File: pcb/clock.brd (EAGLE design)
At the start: 145 x 50 mm, 76 parts, among them IC1 STM32F072C8T6, IC2 REG1117, IC3 24C64ST, SW1 324_SW324_SWITCH_FOOT_HOLE, SW4 324_SW324_SWITCH_FOOT_HOLE, U1 DS18B20, U2 USBC_16P, X2 32.768KHz

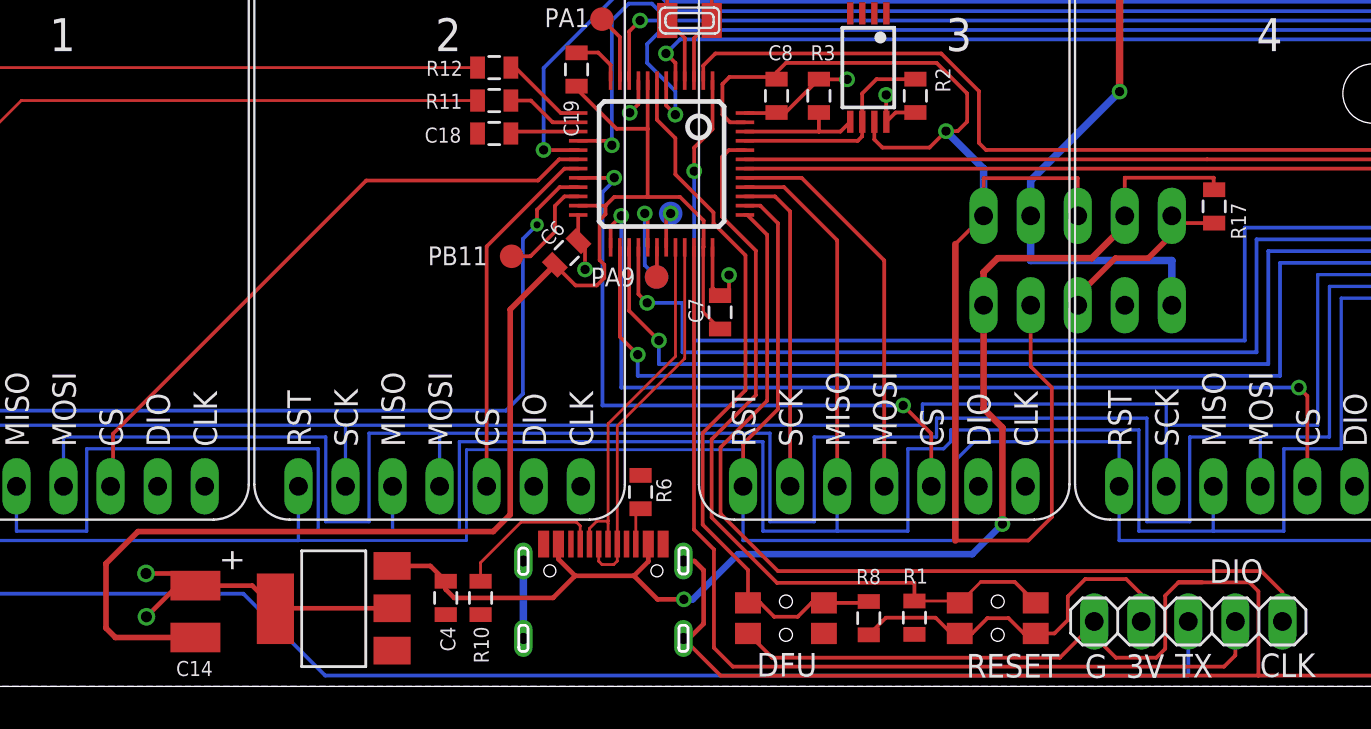
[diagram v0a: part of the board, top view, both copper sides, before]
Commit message: clean up
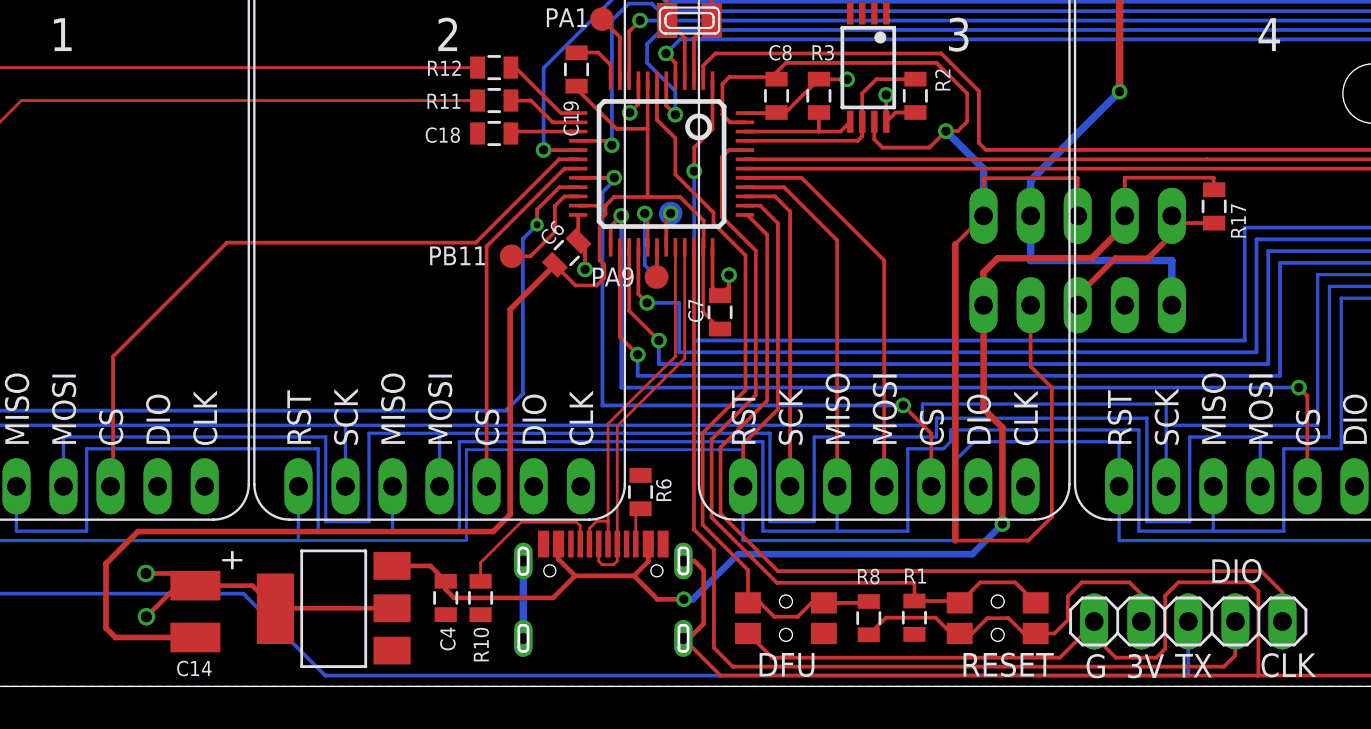
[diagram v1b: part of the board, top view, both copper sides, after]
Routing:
- net EXIXE1_CS: track 34.1 -> 36.6 mm
- net GND: track 277.5 -> 276.2 mm
- net +3V3: track 157.3 -> 156.7 mm
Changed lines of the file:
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@@
 <text x="79.756" y="5.588" size="1.27" layer="25">DIO</text>
 <text x="85.471" y="1.778" size="1.27" layer="25" rot="R180">CLK</text>
-<text x="71.6534" y="1.7526" size="1.27" layer="25" rot="R180">RESET</text>
+<text x="71.3486" y="1.8034" size="1.27" layer="25" rot="R180">RESET</text>
 <text x="58.5724" y="1.8034" size="1.27" layer="25" rot="R180">DFU</text>
 <text x="100.711" y="2.667" size="1.27" layer="25" rot="R180">G</text>
@@
 <contactref element="SW4" pad="P$4"/>
 <contactref element="JP6" pad="1"/>
-<wire x1="78.0796" y1="5.6134" x2="81.915" y2="5.6134" width="0.2032" layer="1"/>
-<wire x1="78.0796" y1="5.6134" x2="77.3684" y2="4.9022" width="0.2032" layer="1"/>
+<wire x1="77.3684" y1="4.9022" x2="78.0796" y2="5.6134" width="0.2032" layer="1"/>
 <wire x1="77.3684" y1="2.032" x2="76.8858" y2="1.5494" width="0.2032" layer="1"/>
 <wire x1="76.8858" y1="1.5494" x2="74.7014" y2="1.5494" width="0.2032" layer="1"/>
@@
 <wire x1="91.96" y1="1.905" x2="90.6392" y2="0.5842" width="0.2032" layer="1"/>
 <wire x1="90.6392" y1="0.5842" x2="82.3976" y2="0.5842" width="0.2032" layer="1"/>
-<wire x1="79.8576" y1="0.5842" x2="53.3645" y2="0.5842" width="0.2032" layer="1"/>
+<wire x1="82.3976" y1="0.5842" x2="53.3645" y2="0.5842" width="0.2032" layer="1"/>
 <wire x1="81.915" y1="5.6134" x2="82.3976" y2="5.1308" width="0.2032" layer="1"/>
 <wire x1="82.3976" y1="5.1308" x2="82.3976" y2="0.5842" width="0.2032" layer="1"/>
 <wire x1="61.666" y1="30.476" x2="61.666" y2="29.52" width="0.2032" layer="1"/>
-<wire x1="78.0796" y1="5.6134" x2="79.375" y2="5.6134" width="0.2032" layer="1"/>
-<wire x1="82.3976" y1="0.5842" x2="79.8576" y2="0.5842" width="0.2032" layer="1"/>
+<wire x1="78.0796" y1="5.6134" x2="81.915" y2="5.6134" width="0.2032" layer="1"/>
 </signal>
 <signal name="+3V3">
@@
 <via x="22.3774" y="3.7592" extent="1-16" drill="0.6"/>
 <via x="53.8226" y="22.1996" extent="1-16" drill="0.5"/>
-<wire x1="53.1622" y1="21.2708" x2="53.34" y2="21.093" width="0.1778" layer="1"/>
 <via x="60.198" y="32.766" extent="1-16" drill="0.5"/>
-<wire x1="54.864" y1="30.948" x2="54.682" y2="30.948" width="0.2032" layer="1"/>
-<wire x1="54.864" y1="30.948" x2="56.359" y2="30.948" width="0.2032" layer="1"/>
+<wire x1="54.682" y1="30.948" x2="56.359" y2="30.948" width="0.2032" layer="1"/>
 <wire x1="56.359" y1="30.948" x2="56.388" y2="30.977" width="0.2032" layer="1"/>
 <wire x1="56.388" y1="30.977" x2="56.874" y2="30.977" width="0.2032" layer="1"/>
@@
 <wire x1="62.2918" y1="3.7084" x2="61.3664" y2="2.783" width="0.2032" layer="1"/>
 <wire x1="76.073" y1="3.5052" x2="76.073" y2="4.9784" width="0.2032" layer="1"/>
-<wire x1="76.073" y1="4.9784" x2="75.2602" y2="5.7912" width="0.2032" layer="1"/>
-<wire x1="73.0504" y1="5.7912" x2="75.2602" y2="5.7912" width="0.2032" layer="1"/>
+<wire x1="76.073" y1="4.9784" x2="75.438" y2="5.6134" width="0.2032" layer="1"/>
+<wire x1="72.8726" y1="5.6134" x2="75.438" y2="5.6134" width="0.2032" layer="1"/>
 <wire x1="25.019" y1="5.4386" x2="24.0568" y2="5.4386" width="0.254" layer="1"/>
 <wire x1="24.0568" y1="5.4386" x2="22.3774" y2="3.7592" width="0.254" layer="1"/>
@@
 <wire x1="60.198" y1="32.766" x2="58.685" y2="32.766" width="0.2032" layer="1"/>
 <wire x1="58.685" y1="32.766" x2="58.674" y2="32.777" width="0.2032" layer="1"/>
-<wire x1="53.8226" y1="22.1996" x2="53.8226" y2="21.093" width="0.2032" layer="1"/>
-<wire x1="53.8226" y1="21.093" x2="53.34" y2="21.093" width="0.2032" layer="1"/>
-<wire x1="52.932" y1="23.698" x2="52.932" y2="21.501" width="0.2032" layer="1"/>
-<wire x1="52.932" y1="21.501" x2="53.34" y2="21.093" width="0.2032" layer="1"/>
 <wire x1="68.9102" y1="3.683" x2="67.7672" y2="3.683" width="0.2032" layer="1"/>
 <wire x1="72.1106" y1="3.5814" x2="72.1106" y2="4.8514" width="0.2032" layer="1"/>
@@
 <wire x1="67.7672" y1="3.683" x2="66.9422" y2="2.858" width="0.2032" layer="1"/>
 <wire x1="66.9422" y1="2.858" x2="66.276" y2="2.858" width="0.2032" layer="1"/>
-<wire x1="72.1106" y1="4.8514" x2="73.0504" y2="5.7912" width="0.2032" layer="1"/>
+<wire x1="72.1106" y1="4.8514" x2="72.8726" y2="5.6134" width="0.2032" layer="1"/>
 <wire x1="143.002" y1="38.618" x2="143.002" y2="13.589" width="0.1524" layer="16"/>
+<wire x1="52.932" y1="23.698" x2="52.932" y2="21.501" width="0.2032" layer="1"/>
+<wire x1="52.932" y1="21.501" x2="53.34" y2="21.093" width="0.2032" layer="1"/>
+<wire x1="53.8226" y1="22.1996" x2="53.8226" y2="21.5756" width="0.2032" layer="1"/>
+<wire x1="53.8226" y1="21.5756" x2="53.34" y2="21.093" width="0.2032" layer="1"/>
 </signal>
 <signal name="N$27">
@@
 <wire x1="56.4134" y1="5.588" x2="63.8302" y2="5.588" width="0.2032" layer="1"/>
 <wire x1="63.8302" y1="5.588" x2="63.8302" y2="4.6084" width="0.2032" layer="1"/>
-<wire x1="69.2452" y1="5.6388" x2="70.376" y2="4.508" width="0.2032" layer="1"/>
-<wire x1="69.2452" y1="5.6388" x2="67.4068" y2="5.6388" width="0.2032" layer="1"/>
-<wire x1="63.8302" y1="4.6084" x2="66.1756" y2="4.6084" width="0.1524" layer="1"/>
-<wire x1="66.1756" y1="4.6084" x2="66.276" y2="4.508" width="0.1524" layer="1"/>
-<wire x1="67.4068" y1="5.6388" x2="66.276" y2="4.508" width="0.1524" layer="1"/>
+<wire x1="69.2706" y1="5.6134" x2="70.376" y2="4.508" width="0.2032" layer="1"/>
+<wire x1="67.3814" y1="5.6134" x2="69.2706" y2="5.6134" width="0.2032" layer="1"/>
+<wire x1="63.8302" y1="4.6084" x2="66.1756" y2="4.6084" width="0.2032" layer="1"/>
+<wire x1="66.1756" y1="4.6084" x2="66.276" y2="4.508" width="0.2032" layer="1"/>
+<wire x1="66.276" y1="4.508" x2="67.3814" y2="5.6134" width="0.2032" layer="1"/>
 </signal>
 <signal name="+5V">
@@
 <contactref element="U$1" pad="CS"/>
 <wire x1="45.682" y1="28.448" x2="44.6532" y2="28.448" width="0.2032" layer="1"/>
-<wire x1="44.6532" y1="28.448" x2="43.5102" y2="27.305" width="0.2032" layer="1"/>
-<wire x1="43.5102" y1="27.305" x2="34.2392" y2="27.305" width="0.2032" layer="1"/>
-<wire x1="34.2392" y1="27.305" x2="20.574" y2="13.6398" width="0.2032" layer="1"/>
-<wire x1="20.574" y1="13.6398" x2="20.574" y2="10.934" width="0.2032" layer="1"/>
+<wire x1="44.6532" y1="28.448" x2="40.1574" y2="23.9522" width="0.2032" layer="1"/>
+<wire x1="40.1574" y1="23.9522" x2="26.7208" y2="23.9522" width="0.2032" layer="1"/>
+<wire x1="26.7208" y1="23.9522" x2="20.574" y2="17.8054" width="0.2032" layer="1"/>
+<wire x1="20.574" y1="17.8054" x2="20.574" y2="10.934" width="0.2032" layer="1"/>
 <wire x1="20.574" y1="10.934" x2="20.44" y2="10.8" width="0.2032" layer="1"/>
 </signal>
@@
 <wire x1="48.932" y1="21.172" x2="49.403" y2="20.701" width="0.2032" layer="1"/>
 <via x="49.403" y="20.701" extent="1-16" drill="0.5"/>
-<wire x1="49.403" y1="20.701" x2="51.308" y2="20.701" width="0.2032" layer="16"/>
-<wire x1="51.308" y1="20.701" x2="51.308" y2="18.034" width="0.2032" layer="16"/>
-<wire x1="51.308" y1="18.034" x2="82.296" y2="18.034" width="0.2032" layer="16"/>
+<wire x1="49.403" y1="20.701" x2="51.1302" y2="20.701" width="0.2032" layer="16"/>
+<wire x1="51.1302" y1="20.701" x2="51.1302" y2="18.034" width="0.2032" layer="16"/>
+<wire x1="51.1302" y1="18.034" x2="82.296" y2="18.034" width="0.2032" layer="16"/>
 <wire x1="82.296" y1="18.034" x2="82.296" y2="24.13" width="0.2032" layer="16"/>
 <wire x1="82.296" y1="24.13" x2="98.806" y2="24.13" width="0.2032" layer="16"/>
